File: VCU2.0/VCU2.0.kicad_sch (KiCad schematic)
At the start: 4 parts

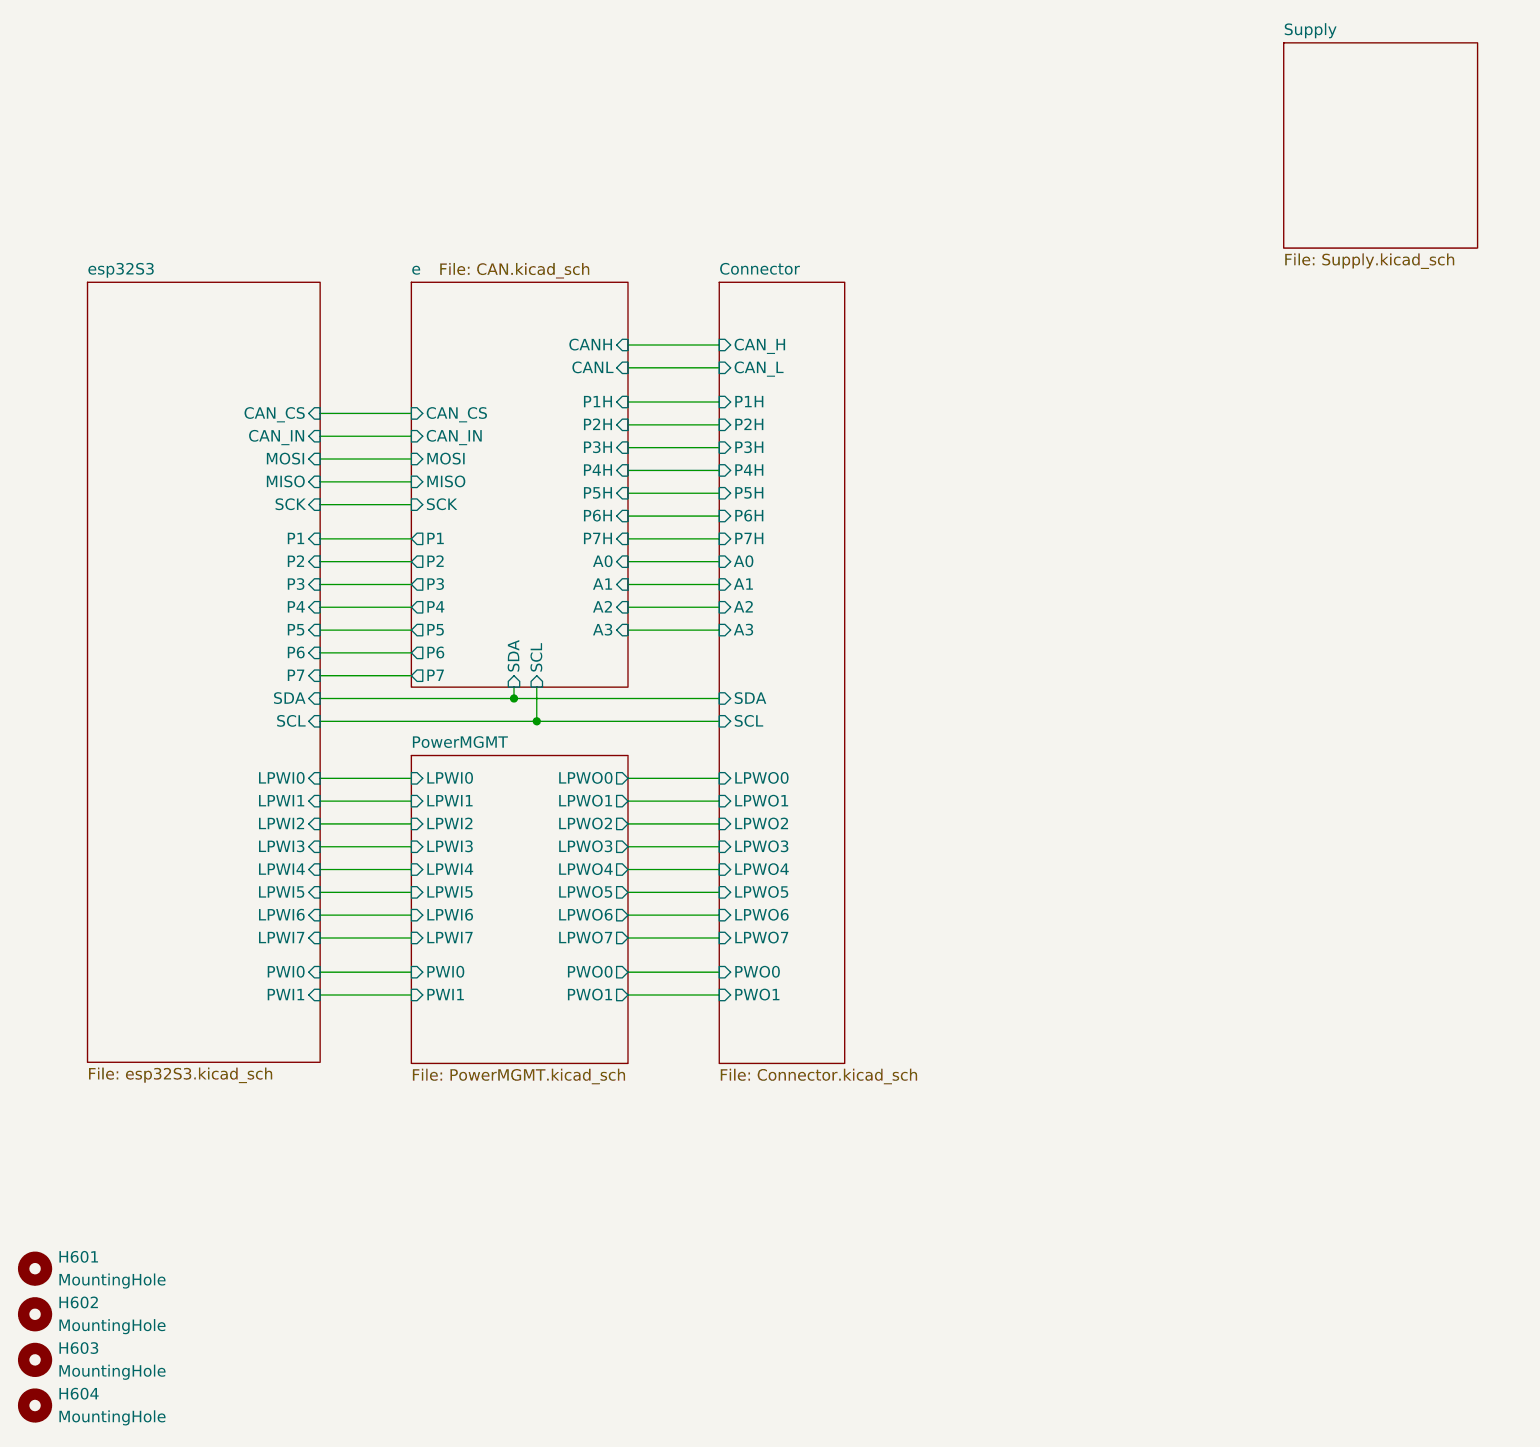
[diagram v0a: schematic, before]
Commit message: simple regen
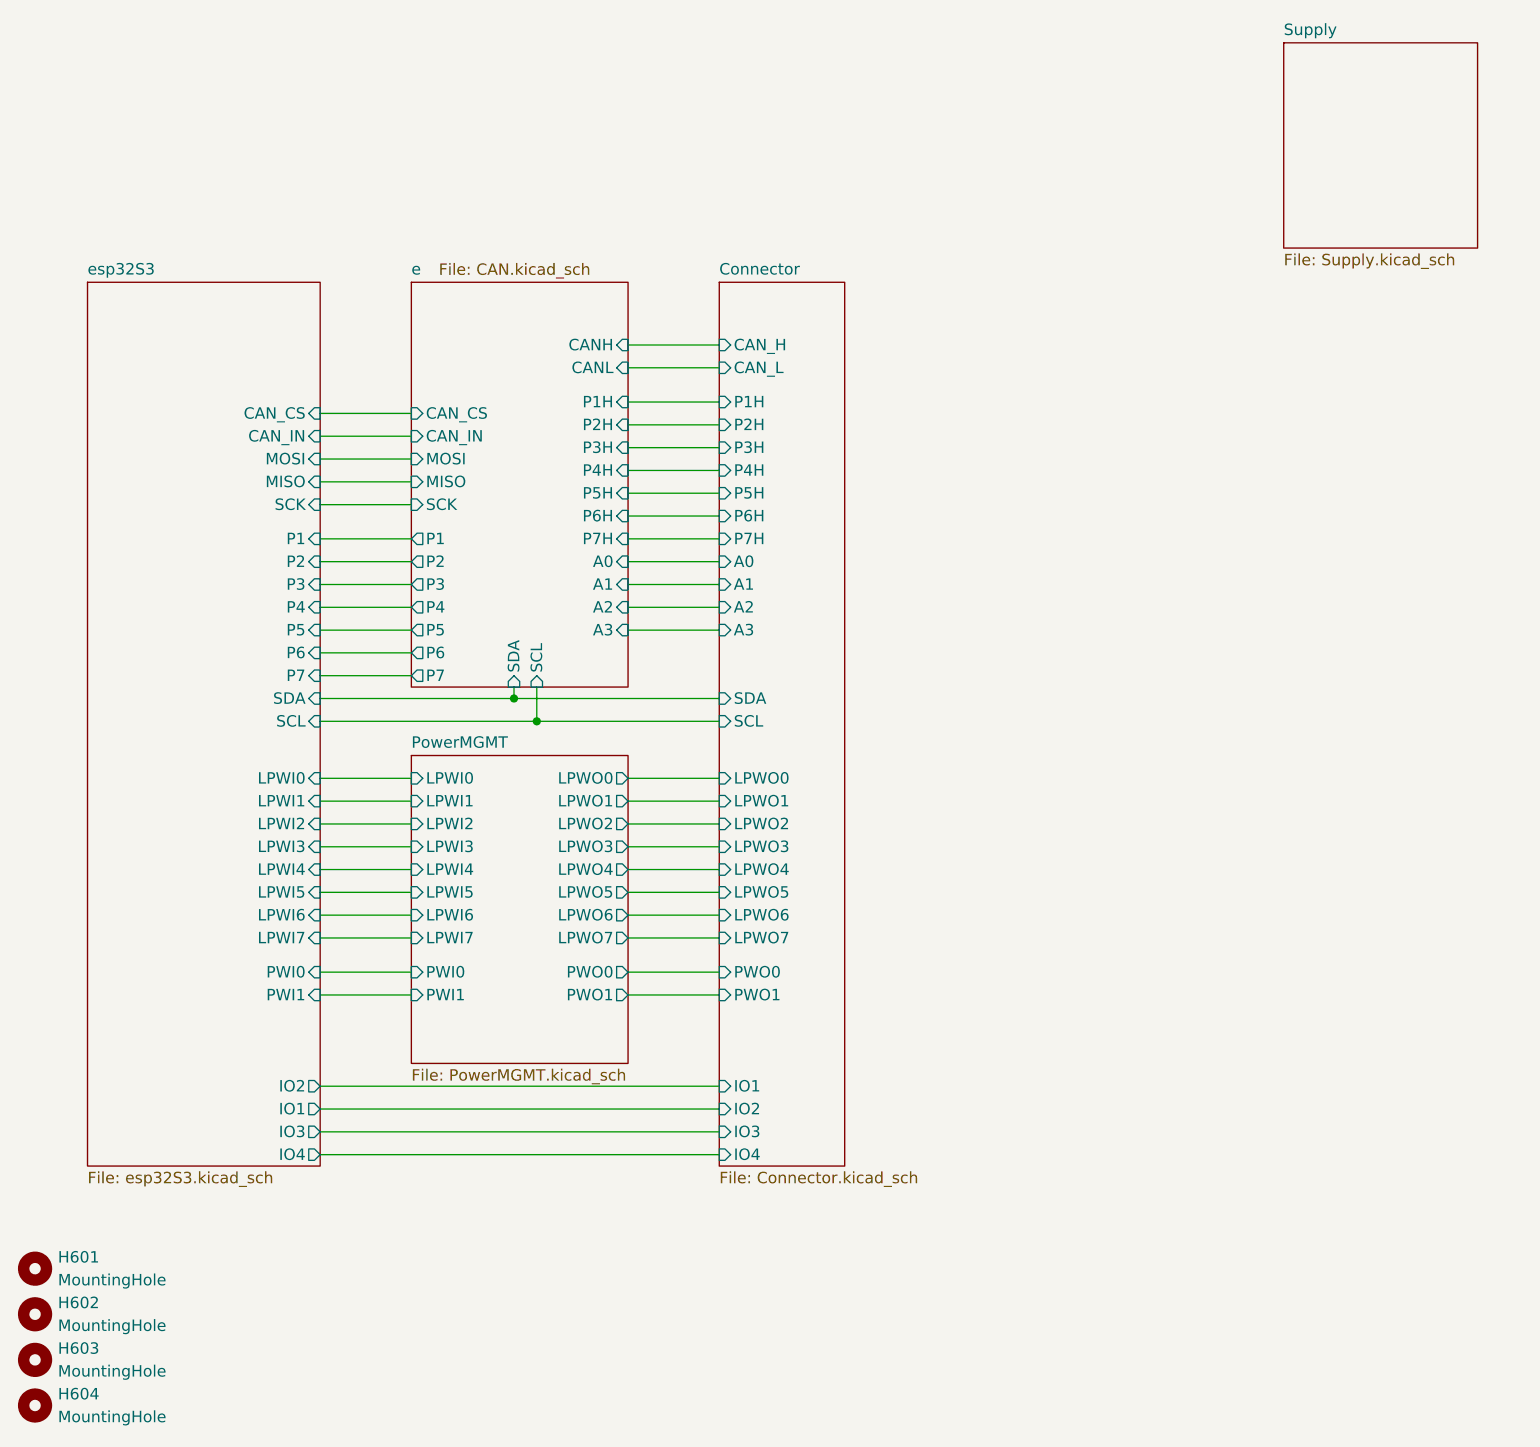
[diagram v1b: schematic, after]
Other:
- sheet Connector ports: added IO1, IO2, IO3, IO4; removed none
- sheet esp32S3 ports: added IO1, IO2, IO3, IO4; removed none
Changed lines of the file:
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@@
+	(wire
+		(pts
+			(xy 130.81 146.05) (xy 175.26 146.05)
+		)
+		(stroke
+			(width 0)
+			(type default)
+		)
+	)
 	(wire
 		(pts
@@
 	(wire
 		(pts
+			(xy 130.81 138.43) (xy 175.26 138.43)
+		)
+		(stroke
+			(width 0)
+			(type default)
+		)
+	)
+	(wire
+		(pts
+			(xy 130.81 140.97) (xy 175.26 140.97)
+		)
+		(stroke
+			(width 0)
+			(type default)
+		)
+	)
+	(wire
+		(pts
 			(xy 130.81 95.25) (xy 152.4 95.25)
 		)
@@
 		(pts
 			(xy 165.1 58.42) (xy 175.26 58.42)
+		)
+		(stroke
+			(width 0)
+			(type default)
+		)
+	)
+	(wire
+		(pts
+			(xy 130.81 143.51) (xy 175.26 143.51)
 		)
 		(stroke
@@
 	(sheet
 		(at 175.26 48.895)
-		(size 13.97 86.995)
+		(size 13.97 98.425)
 		(fields_autoplaced yes)
 		(stroke
@@
 		)
 		(property "Sheetfile" "Connector.kicad_sch"
-			(at 175.26 136.4746 0)
+			(at 175.26 147.9046 0)
 			(effects
 				(font
@@
 		(pin "PWO0" input
 			(at 175.26 125.73 180)
+			(effects
+				(font
+					(size 1.27 1.27)
+				)
+				(justify left)
+			)
+		)
+		(pin "IO1" input
+			(at 175.26 138.43 180)
+			(effects
+				(font
+					(size 1.27 1.27)
+				)
+				(justify left)
+			)
+		)
+		(pin "IO2" input
+			(at 175.26 140.97 180)
+			(effects
+				(font
+					(size 1.27 1.27)
+				)
+				(justify left)
+			)
+		)
+		(pin "IO3" input
+			(at 175.26 143.51 180)
+			(effects
+				(font
+					(size 1.27 1.27)
+				)
+				(justify left)
+			)
+		)
+		(pin "IO4" input
+			(at 175.26 146.05 180)
 			(effects
 				(font
@@
 	(sheet
 		(at 104.902 48.895)
-		(size 25.908 86.868)
+		(size 25.908 98.425)
 		(fields_autoplaced yes)
 		(stroke
@@
 		)
 		(property "Sheetfile" "esp32S3.kicad_sch"
-			(at 104.902 136.3476 0)
+			(at 104.902 147.9046 0)
 			(effects
 				(font
@@
 			(effects
 				(font
+					(size 1.27 1.27)
+				)
+				(justify right)
+			)
+		)
+		(pin "IO2" output
+			(at 130.81 138.43 0)
+			(effects
+				(font
+					(size 1.27 1.27)
+				)
+				(justify right)
+			)
+		)
+		(pin "IO1" output
+			(at 130.81 140.97 0)
+			(effects
+				(font
+					(size 1.27 1.27)
+				)
+				(justify right)
+			)
+		)
+		(pin "IO3" output
+			(at 130.81 143.51 0)
+			(effects
+				(font
+					(size 1.27 1.27)
+				)
+				(justify right)
+			)
+		)
+		(pin "IO4" output
+			(at 130.81 146.05 0)
+			(effects
+				(font
